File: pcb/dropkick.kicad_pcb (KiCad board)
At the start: 2 copper layers, 44.5 x 50.8 mm, 51 parts, among them SW1 CONN3_020524_WRE, SW2 KMR211NG_LFS, U1 ATSAMD21G18A-AUT, U2 SAM-M8Q-0-10, U3 MCP73831T-2ACI/OT, U4 DPS310, U5 MPU-6050, U6 SPX3819-3.3, X1 microUSB, X2 JSTPH, X3 microsd, X5 32768Hz

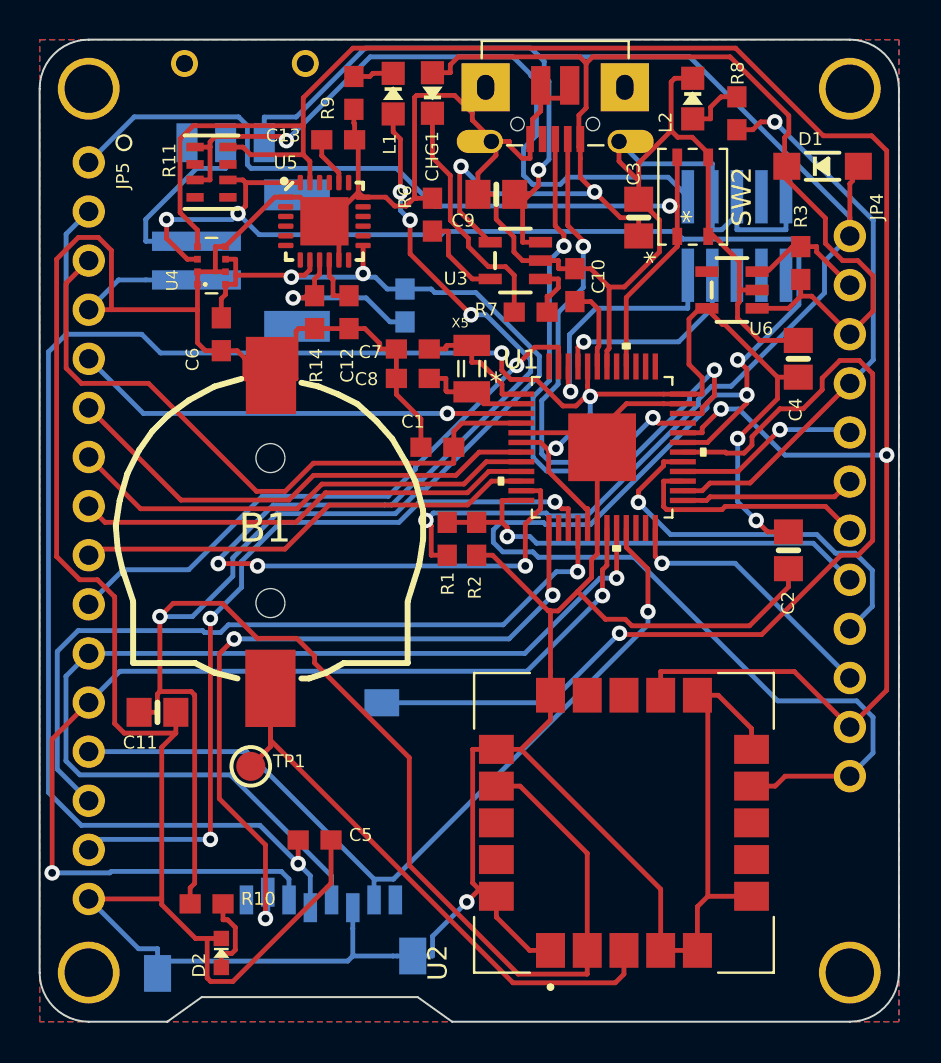
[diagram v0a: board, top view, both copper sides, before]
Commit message: V2-SAM working draft
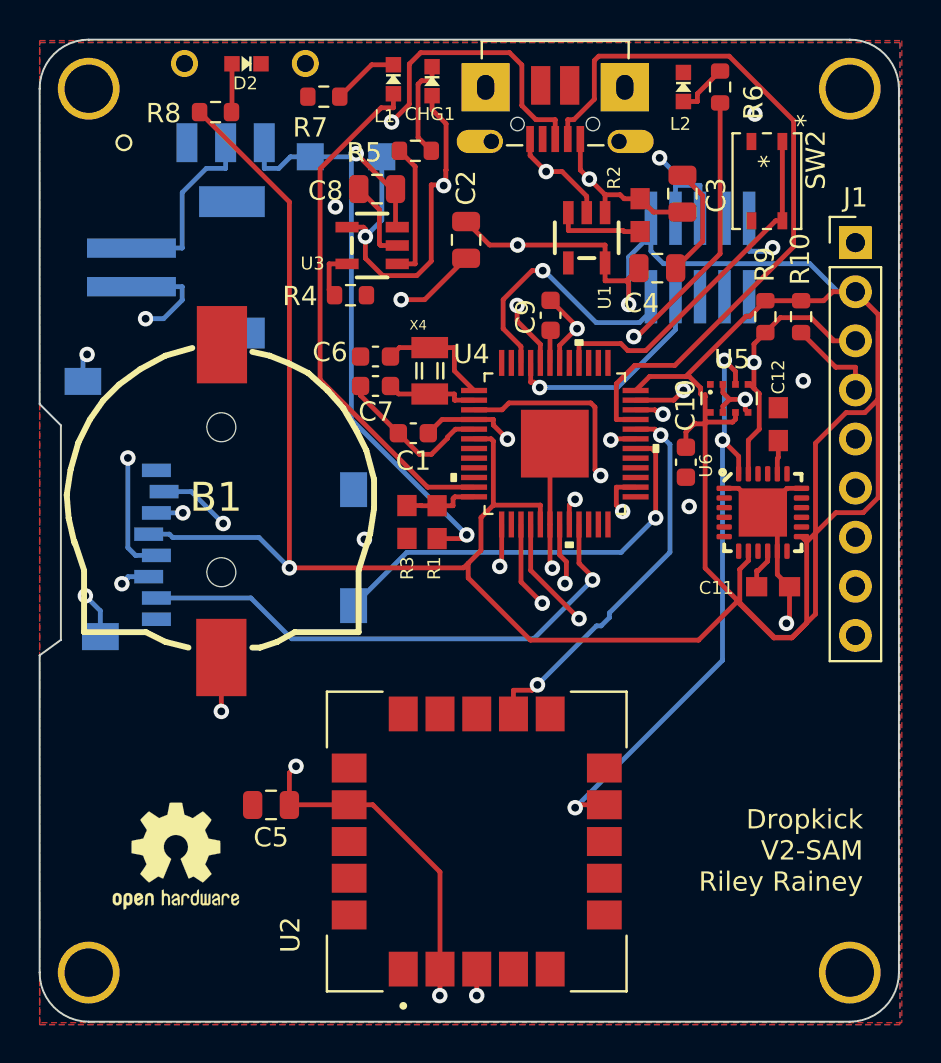
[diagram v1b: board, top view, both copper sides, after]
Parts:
- removed the C5 at (77.7, 85.9)
- removed JP2: 20021221-00010C4LF, lib_fr:3221-10-0300-00-TR
- removed JP4: HEADER-1X12, lib_fr:1X12_ROUND
- removed JP5: HEADER-1X16ROUND, lib_fr:1X16_ROUND
- removed R11: 4.7K, lib_fr:RESPACK_4X0603
- removed R14: 10K, lib_fr:0603-NO
- removed SJ4: SOLDERJUMPER, lib_fr:0603-NO
- removed TP1: TESTPOINTROUND1.5MM, lib_fr:TESTPOINT_ROUND_1.5MM
- removed X5: 32768Hz, lib_fr:XTAL3215
- added J1: Conn_01x08, Connector_PinHeader_2.54mm:PinHeader_1x09_P2.54mm_Vertical, F.Cu at (105.7, 55.0)
- added JP1: 3221-10-0300-00-TR, lib_fr:3221-10-0300-00-TR, B.Cu at (97.7, 55.7)
- added R4: 10K, Resistor_SMD:R_0603_1608Metric, F.Cu at (79.6, 57.7)
- added R5: 1K, Resistor_SMD:R_0603_1608Metric, F.Cu at (82.9, 50.2)
- added REF2: OSHW-Logo2_7.3x6mm_SilkScreen, Symbol:OSHW-Logo2_7.3x6mm_SilkScreen, F.Cu at (70.5, 86.7)
- added X4: 32768Hz, lib_fr:XTAL3215, F.Cu at (83.7, 61.6)
- C1: footprint lib_fr:0603-NO -> Capacitor_SMD:C_0603_1608Metric
- C10: renamed from C11; value 10uF -> 0.1uF; footprint lib_fr:0805-NO -> Capacitor_SMD:C_0603_1608Metric
- C2, C3, C4: footprint lib_fr:0805-NO -> Capacitor_SMD:C_0805_2012Metric
- C5: renamed from C6; value 0.1uF -> 10uF; footprint lib_fr:0603-NO -> Capacitor_SMD:C_0805_2012Metric
- C6: renamed from C7; footprint lib_fr:0603-NO -> Capacitor_SMD:C_0603_1608Metric
- C7: renamed from C8; footprint lib_fr:0603-NO -> Capacitor_SMD:C_0603_1608Metric
- C8: renamed from C9; footprint lib_fr:0805-NO -> Capacitor_SMD:C_0805_2012Metric
- C9: renamed from C10; footprint lib_fr:0603-NO -> Capacitor_SMD:C_0603_1608Metric
- CHG1, L1, L2: footprint lib_fr:CHIPLED_0805_NOOUTLINE -> lib_fr:CHIPLED_0603_NOOUTLINE
- D1: moved to B.Cu
- R10, R7: footprint lib_fr:0603-NO -> Resistor_SMD:R_0603_1608Metric
- R2: value 100K -> 100k
- R3: value 100k -> 100K
- R6: value 10K -> 2.2K; footprint lib_fr:0603-NO -> Resistor_SMD:R_0603_1608Metric
- R8: value 2.2K -> 10K; footprint lib_fr:0603-NO -> Resistor_SMD:R_0603_1608Metric
- R9: value 1K -> 10K; footprint lib_fr:0603-NO -> Resistor_SMD:R_0603_1608Metric
- SW1: value CONN3_020524_WRE -> 450405020524
- U1: value ATSAMD21G18A-AUT -> SPX3819-3.3; footprint lib_fr:ATSAMD21G15B-AU -> lib_fr:SOT23-5
- U4: value DPS310 -> ATSAMD21G18A-AUT; footprint lib_fr:DPS310XTSA1 -> lib_fr:ATSAMD21G15B-AU
- U5: value MPU-6050 -> DPS310XTSA1; footprint lib_fr:QFN24_4MM_SMSC -> lib_fr:DPS310XTSA1
- U6: value SPX3819-3.3 -> MPU-6050; footprint lib_fr:SOT23-5 -> lib_fr:QFN24_4MM_SMSC
- moved D2 46.0 mm to (74.2, 45.7), turned to -90 degrees
- moved R10 43.2 mm to (102.9, 58.8), turned to -90 degrees
- moved C10 30.2 mm to (96.9, 66.3), turned to -90 degrees
- moved C12 27.1 mm to (101.7, 64.3), turned to 90 degrees
- moved R8 27.0 mm to (72.6, 48.2), turned to 0 degrees
- moved C11 26.1 mm to (101.4, 72.8), turned to 0 degrees
- moved D1 24.7 mm to (79.3, 50.5), turned to 180 degrees
- moved C5 24.5 mm to (75.5, 84.0), turned to 180 degrees
- moved R3 24.4 mm to (82.5, 69.4), turned to -90 degrees
- moved R9 24.2 mm to (101.0, 58.8)
- moved C2 23.1 mm to (85.6, 54.8)
- moved U5 22.9 mm to (99.2, 63.0)
- moved U4 20.0 mm to (90.2, 65.3), turned to 0 degrees
- moved R2 18.8 mm to (94.6, 53.5)
- moved R6 16.3 mm to (98.7, 46.9)
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- renumbered C12 to C11, C13 to C12, REF** to REF1
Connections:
- C10 pad 1: 3.3V -> +3V3
- C5 pad 1: 3.3V -> +3V3
- C6 pad 1: Net-(C7-Pad1) -> Net-(C6-Pad1)
- C7 pad 1: Net-(C8-Pad1) -> Net-(C7-Pad1)
- C9 pad 1: Net-(C10-Pad1) -> Net-(C9-Pad1)
- R10 pad 1: 3.3V -> +3V3
- R10 pad 2: Net-(D2-PadA) -> /SDA
- R2 pad 1: /D9 -> VBUS
- R2 pad 2: GND -> /EN
- R3 pad 1: VBUS -> /D9
- R3 pad 2: /EN -> GND
- R6 pad 1: Net-(R6-Pad1) -> /D13
- R6 pad 2: GND -> Net-(L2-PadA)
- R7 pad 1: Net-(CHG1-PadC) -> Net-(L1-PadC)
- R7 pad 2: Net-(R7-Pad2) -> GND
- R8 pad 1: /D13 -> +3V3
- R8 pad 2: Net-(L2-PadA) -> Net-(D2-PadA)
- R9 pad 1: Net-(L1-PadC) -> +3V3
- R9 pad 2: GND -> /SCL
- U1 pad 1: Net-(C7-Pad1) -> VBUS
- U1 pad 2: Net-(C8-Pad1) -> GND
- U1 pad 3: /A0 -> /EN
- U1 pad 4: /AREF -> unconnected-(U1-Pad4)
- U1 pad 5: GND -> +3V3
- U2 pad 17: 3.3V -> +3V3
- U2 pad 2: 3.3V -> +3V3
- U3 pad 1: Net-(R7-Pad2) -> Net-(R5-Pad2)
- U3 pad 5: Net-(R6-Pad1) -> Net-(R4-Pad1)
- U4 pad 1: GND -> Net-(C6-Pad1)
- U4 pad 2: GND -> Net-(C7-Pad1)
- U4 pad 3: /SDA -> /A0
- U4 pad 4: /SCL -> /AREF
- U4 pad 6: 3.3V -> +3V3
- U4 pad 7: GND -> /A1
- U4 pad 8: 3.3V -> /A2
- U5 pad 2: (no net) -> GND
- U5 pad 3: (no net) -> /SDA
- U5 pad 4: (no net) -> /SCL
- U5 pad 5: (no net) -> GND
- U5 pad 6: /SDA_EXT -> +3V3
- U5 pad 7: /SCL_EXT -> GND
- U5 pad 8: 3.3V -> +3V3
- U6 pad 1: VBUS -> GND
- U6 pad 2: GND -> (no net)
- U6 pad 3: /EN -> (no net)
- U6 pad 4: unconnected-(U6-Pad4) -> (no net)
- U6 pad 5: +3V3 -> (no net)
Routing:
- net GND: track 337.6 -> 75.3 mm, vias 1 -> 18
- net 3.3V: track 116.2 -> 0.00 mm, vias 3 -> 0
- net +3V3: track 118.3 -> 230.0 mm
- net /SCL: track 109.6 -> 40.3 mm, vias 2 -> 3
- net /SDA: track 105.4 -> 51.7 mm
- net VCC: track 37.4 -> 0.00 mm, vias 1 -> 0
- net /D8: track 58.3 -> 27.0 mm, vias 6 -> 0
- net /A5: track 30.9 -> 0.00 mm, vias 1 -> 0
- net /MOSI: track 55.6 -> 26.0 mm
- net /D7: track 50.3 -> 22.0 mm
- net /~{RESET}: track 46.6 -> 18.6 mm, vias 1 -> 0
- net VBUS: track 65.1 -> 37.1 mm, vias 2 -> 3
- net /A1: track 25.4 -> 0.00 mm
- net /A2: track 24.5 -> 0.00 mm
- net /A4: track 24.0 -> 0.00 mm
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- added copper zone on In1.Cu, net GND
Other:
- outline, holes or cut-outs redrawn
- copper layers 2 -> 4
- board text added: "+3.3"
- board text added: "A0"
- board text added: "AREF"
- board text added: "D0"
- board text added: "D1"
- board text added: "Dropkick V2-SAM Copyright (c) 2022 Riley Rainey https://GitHub.com/rrainey/dropkick/"
- board text added: "Dropkick V2-SAM Riley Rainey"
- board text added: "GND"
- board text added: "SCL"
- board text added: "SDA"
- board text added: "VBAT"
- board text removed: "Dropkick V1 Copyright (c) 2022 Riley Rainey https://GitHub.com/rrainey/dropkick/"
